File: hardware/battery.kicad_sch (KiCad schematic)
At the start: 12 parts, among them IC1 BQ29732DSER, Q1 CSD16406Q3, Q2 CSD16406Q3

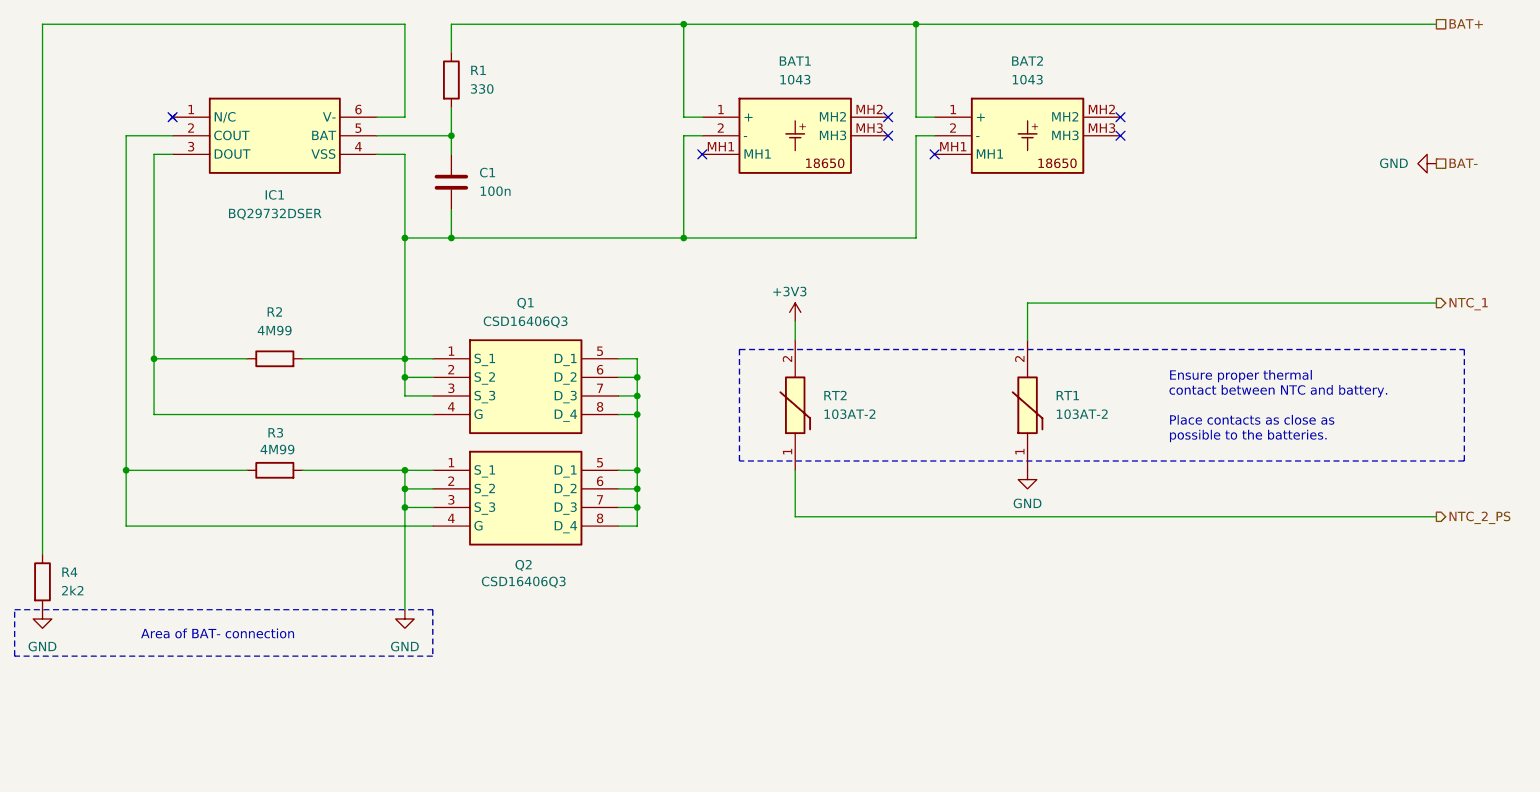
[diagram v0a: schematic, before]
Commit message: Revised and completed BOM
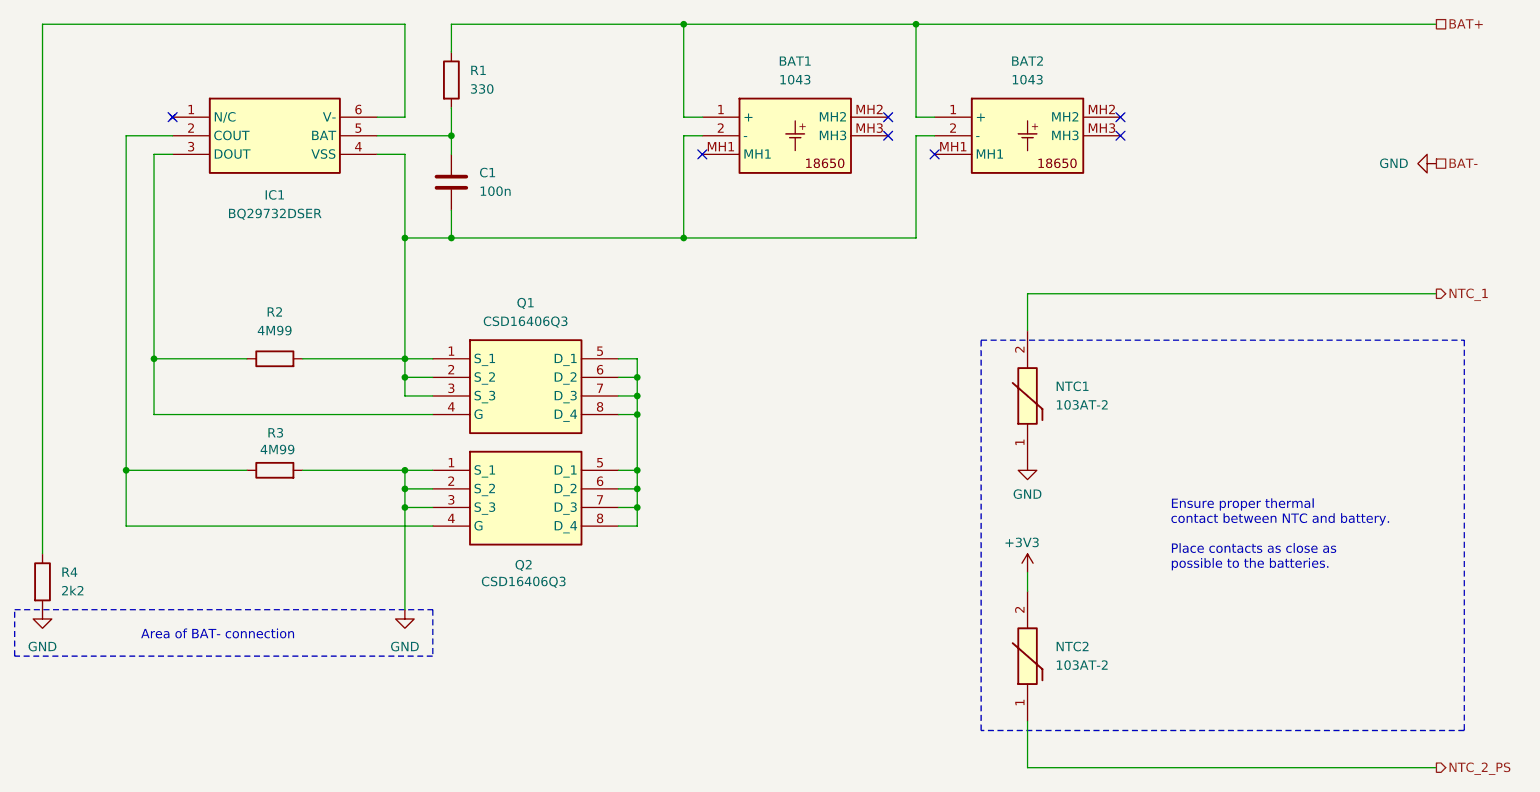
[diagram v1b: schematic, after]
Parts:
- R2, R3: footprint Resistor_SMD:R_0805_2012Metric -> Resistor_SMD:R_0402_1005Metric
- renumbered RT1 to NTC1, RT2 to NTC2
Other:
- moved on the sheet: NTC1, NTC2
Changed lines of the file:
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@@
 	(wire
 		(pts
-			(xy 157.48 97.79) (xy 157.48 100.33)
+			(xy 189.23 132.08) (xy 189.23 134.62)
 		)
 		(stroke
@@
 	(wire
 		(pts
+			(xy 189.23 158.75) (xy 245.11 158.75)
+		)
+		(stroke
+			(width 0)
+			(type default)
+		)
+	)
+	(wire
+		(pts
 			(xy 135.89 125.73) (xy 135.89 123.19)
 		)
@@
 	(wire
 		(pts
-			(xy 189.23 95.25) (xy 189.23 100.33)
+			(xy 189.23 93.98) (xy 189.23 99.06)
 		)
 		(stroke
@@
 	(wire
 		(pts
-			(xy 245.11 124.46) (xy 157.48 124.46)
-		)
-		(stroke
-			(width 0)
-			(type default)
-		)
-	)
-	(wire
-		(pts
 			(xy 69.85 102.87) (xy 82.55 102.87)
 		)
@@
 	(wire
 		(pts
-			(xy 245.11 95.25) (xy 189.23 95.25)
+			(xy 245.11 93.98) (xy 189.23 93.98)
 		)
 		(stroke
@@
 	(wire
 		(pts
-			(xy 157.48 124.46) (xy 157.48 118.11)
+			(xy 189.23 158.75) (xy 189.23 152.4)
 		)
 		(stroke
@@
 	)
 	(rectangle
-		(start 149.86 101.6)
-		(end 248.92 116.84)
+		(start 182.88 100.33)
+		(end 248.92 153.67)
 		(stroke
 			(width 0)
@@
 	(text "Ensure proper thermal \ncontact between NTC and battery.\n\nPlace contacts as close as \npossible to the batteries."
 		(exclude_from_sim no)
-		(at 208.534 109.474 0)
+		(at 208.788 127 0)
 		(effects
 			(font
@@
 	(hierarchical_label "NTC_2_PS"
 		(shape output)
-		(at 245.11 124.46 0)
+		(at 245.11 158.75 0)
 		(effects
 			(font
@@
 	(hierarchical_label "NTC_1"
 		(shape output)
-		(at 245.11 95.25 0)
+		(at 245.11 93.98 0)
 		(effects
 			(font
@@
 	(symbol
 		(lib_id "SamacSys_Parts:103AT-2")
-		(at 157.48 118.11 90)
+		(at 189.23 152.4 90)
 		(unit 1)
 		(exclude_from_sim no)
@@
 		(dnp no)
 		(fields_autoplaced yes)
-		(property "Reference" "RT2"
-			(at 161.29 107.9499 90)
+		(property "Reference" "NTC2"
+			(at 193.04 142.2399 90)
 			(effects
 				(font
@@
 		)
 		(property "Value" "103AT-2"
-			(at 161.29 110.4899 90)
+			(at 193.04 144.7799 90)
 			(effects
 				(font
@@
 		)
 		(property "Footprint" "103AT2"
-			(at 253.67 104.14 0)
+			(at 285.42 138.43 0)
 			(effects
 				(font
@@
 		)
 		(property "Datasheet" "https://www.semitec-global.com/uploads/2022/01/P12-13-AT-Thermistor.pdf"
-			(at 353.67 104.14 0)
+			(at 385.42 138.43 0)
 			(effects
 				(font
@@
 		)
 		(property "Description" "NTC (Negative Temperature Coefficient) Thermistors 10kohm 1%"
-			(at 157.48 118.11 0)
+			(at 189.23 152.4 0)
 			(effects
 				(font
@@
 		)
 		(property "Height" "9.5"
-			(at 553.67 104.14 0)
+			(at 585.42 138.43 0)
 			(effects
 				(font
@@
 		)
 		(property "Manufacturer_Name" "Semitec"
-			(at 653.67 104.14 0)
+			(at 685.42 138.43 0)
 			(effects
 				(font
@@
 		)
 		(property "Manufacturer_Part_Number" "103AT-2"
-			(at 753.67 104.14 0)
+			(at 785.42 138.43 0)
 			(effects
 				(font
@@
 		)
 		(property "Mouser Part Number" "954-103AT-2"
-			(at 853.67 104.14 0)
+			(at 885.42 138.43 0)
 			(effects
 				(font
@@
 		)
 		(property "Mouser Price/Stock" "https://www.mouser.co.uk/ProductDetail/Semitec/103AT-2?qs=wgO0AD0o1vvcDzsKguD%252Bew%3D%3D"
-			(at 953.67 104.14 0)
+			(at 985.42 138.43 0)
 			(effects
 				(font
@@
 		)
 		(property "Arrow Part Number" ""
-			(at 1053.67 104.14 0)
+			(at 1085.42 138.43 0)
 			(effects
 				(font
@@
 		)
 		(property "Arrow Price/Stock" ""
-			(at 1153.67 104.14 0)
+			(at 1185.42 138.43 0)
 			(effects
 				(font
@@
 			(project "obvod"
 				(path "/e8e834c4-1afb-42f7-b718-3cb720dae1d5/f61c7da5-11ee-4b50-a688-248a75ac3e8f"
-					(reference "RT2")
+					(reference "NTC2")
 					(unit 1)
 				)
@@
 	(symbol
 		(lib_id "power:GND")
-		(at 189.23 118.11 0)
+		(at 189.23 116.84 0)
 		(unit 1)
 		(exclude_from_sim no)
@@
 		(dnp no)
 		(property "Reference" "#PWR073"
-			(at 189.23 124.46 0)
+			(at 189.23 123.19 0)
 			(effects
 				(font
@@
 		)
 		(property "Value" "GND"
-			(at 189.23 122.682 0)
+			(at 189.23 121.412 0)
 			(effects
 				(font
@@
 		)
 		(property "Footprint" ""
-			(at 189.23 118.11 0)
+			(at 189.23 116.84 0)
 			(effects
 				(font
@@
 		)
 		(property "Datasheet" ""
-			(at 189.23 118.11 0)
+			(at 189.23 116.84 0)
 			(effects
 				(font
@@
 		)
 		(property "Description" "Power symbol creates a global label with name \"GND\" , ground"
-			(at 189.23 118.11 0)
+			(at 189.23 116.84 0)
 			(effects
 				(font
@@
 			)
 		)
-		(property "Footprint" "Resistor_SMD:R_0805_2012Metric"
+		(property "Footprint" "Resistor_SMD:R_0402_1005Metric"
 			(at 86.36 119.888 90)
 			(effects
@@
 	(symbol
 		(lib_id "SamacSys_Parts:103AT-2")
-		(at 189.23 118.11 90)
+		(at 189.23 116.84 90)
 		(unit 1)
 		(exclude_from_sim no)
@@
 		(dnp no)
 		(fields_autoplaced yes)
-		(property "Reference" "RT1"
-			(at 193.04 107.9499 90)
+		(property "Reference" "NTC1"
+			(at 193.04 106.6799 90)
 			(effects
 				(font
@@
 		)
 		(property "Value" "103AT-2"
-			(at 193.04 110.4899 90)
+			(at 193.04 109.2199 90)
 			(effects
 				(font
@@
 		)
 		(property "Footprint" "103AT2"
-			(at 285.42 104.14 0)
+			(at 285.42 102.87 0)
 			(effects
 				(font
@@
 		)
 		(property "Datasheet" "https://www.semitec-global.com/uploads/2022/01/P12-13-AT-Thermistor.pdf"
-			(at 385.42 104.14 0)
+			(at 385.42 102.87 0)
 			(effects
 				(font
@@
 		)
 		(property "Description" "NTC (Negative Temperature Coefficient) Thermistors 10kohm 1%"
-			(at 189.23 118.11 0)
+			(at 189.23 116.84 0)
 			(effects
 				(font
@@
 		)
 		(property "Height" "9.5"
-			(at 585.42 104.14 0)
+			(at 585.42 102.87 0)
 			(effects
 				(font
@@
 		)
 		(property "Manufacturer_Name" "Semitec"
-			(at 685.42 104.14 0)
+			(at 685.42 102.87 0)
 			(effects
 				(font
@@
 		)
 		(property "Manufacturer_Part_Number" "103AT-2"
-			(at 785.42 104.14 0)
+			(at 785.42 102.87 0)
 			(effects
 				(font
@@
 		)
 		(property "Mouser Part Number" "954-103AT-2"
-			(at 885.42 104.14 0)
+			(at 885.42 102.87 0)
 			(effects
 				(font
@@
 		)
 		(property "Mouser Price/Stock" "https://www.mouser.co.uk/ProductDetail/Semitec/103AT-2?qs=wgO0AD0o1vvcDzsKguD%252Bew%3D%3D"
-			(at 985.42 104.14 0)
+			(at 985.42 102.87 0)
 			(effects
 				(font
@@
 		)
 		(property "Arrow Part Number" ""
-			(at 1085.42 104.14 0)
+			(at 1085.42 102.87 0)
 			(effects
 				(font
@@
 		)
 		(property "Arrow Price/Stock" ""
-			(at 1185.42 104.14 0)
+			(at 1185.42 102.87 0)
 			(effects
 				(font
@@
 			(project "obvod"
 				(path "/e8e834c4-1afb-42f7-b718-3cb720dae1d5/f61c7da5-11ee-4b50-a688-248a75ac3e8f"
-					(reference "RT1")
+					(reference "NTC1")
 					(unit 1)
 				)
@@
 			)
 		)
-		(property "Footprint" "Resistor_SMD:R_0805_2012Metric"
+		(property "Footprint" "Resistor_SMD:R_0402_1005Metric"
 			(at 86.36 104.648 90)
 			(effects
@@
 	(symbol
 		(lib_id "power:+3V3")
-		(at 157.48 97.79 0)
+		(at 189.23 132.08 0)
 		(unit 1)
 		(exclude_from_sim no)
@@
 		(dnp no)
 		(property "Reference" "#PWR072"
-			(at 157.48 101.6 0)
+			(at 189.23 135.89 0)
 			(effects
 				(font
@@
 		)
 		(property "Value" "+3V3"
-			(at 156.718 93.726 0)
+			(at 188.468 128.016 0)
 			(effects
 				(font
@@
 		)
 		(property "Footprint" ""
-			(at 157.48 97.79 0)
+			(at 189.23 132.08 0)
 			(effects
 				(font
@@
 		)
 		(property "Datasheet" ""
-			(at 157.48 97.79 0)
+			(at 189.23 132.08 0)
 			(effects
 				(font
@@
 		)
 		(property "Description" "Power symbol creates a global label with name \"+3V3\""
-			(at 157.48 97.79 0)
-			(effects
-				(font
+			(at 189.23 132.08 0)
+			(effects
+				(font
